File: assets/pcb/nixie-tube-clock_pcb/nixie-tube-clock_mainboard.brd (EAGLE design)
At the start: 90.2 x 40.6 mm, 14 parts, among them J1 POW (5V), P1 MX, P2 MXX, P3 HX, P4 HXX, P7 RTC, P8 HV_EN

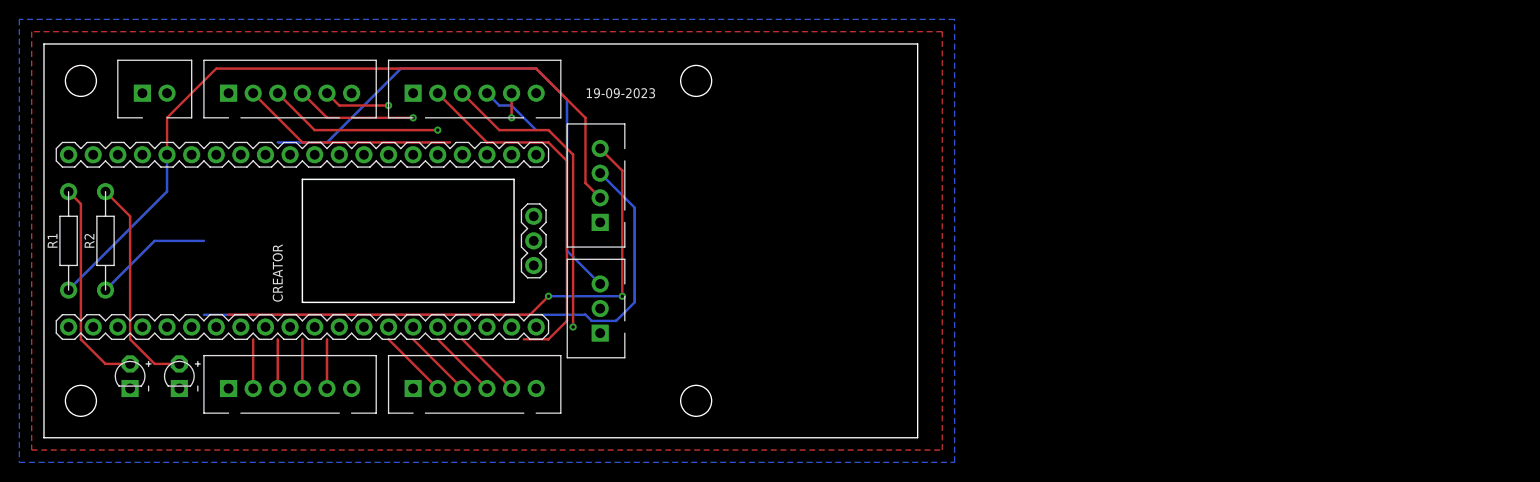
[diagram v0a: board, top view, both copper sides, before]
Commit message: cleaned up files
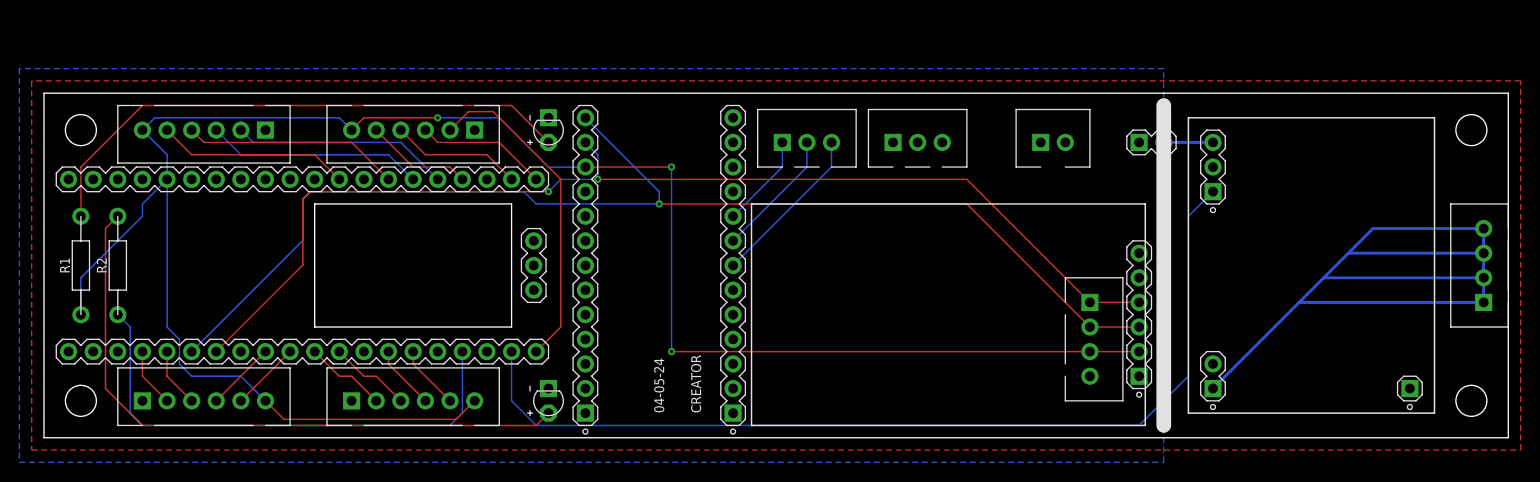
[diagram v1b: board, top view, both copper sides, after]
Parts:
- added GND: GND, myLibrary:XH2.54_3-PIN
- added JP1: (no value), myLibrary:HEADER_2-PIN_JUMPER
- added P11: CAP1188, myLibrary:HEADER_13-PIN
- added P12: (no value), myLibrary:HEADER_13-PIN
- added P5: RTC_A, myLibrary:HEADER_6-PIN
- added P6: HV_OUT, myLibrary:HEADER_2-PIN
- added P9: HV_OUT, myLibrary:XH2.54_4-PIN
- added RTC_B: RTC_B, myLibrary:XH2.54_4-PIN
- added TOUCH: TOUCH, myLibrary:XH2.54_3-PIN
- CREATOR: value Isaac -> ISAAC
- P1: value MX -> MXX
- P2: value MXX -> MX
- P3: value HX -> HXX
- P4: value HXX -> HX
- P7: value RTC -> HV_IN; device myLibrary:XH2.54_4-PIN -> myLibrary:HEADER_3-PIN
- P8: value HV_EN -> (none); device myLibrary:XH2.54_3-PIN -> myLibrary:HEADER_1-PIN
- SCHEMATIC1: value 19-09-2023 -> 04-05-24
- moved J1 92.8 mm to (104.1, 30.5)
- moved P8 84.0 mm to (141.0, 5.08), turned to 0 degrees
- moved P7 63.2 mm to (120.7, 25.4), turned to 0 degrees
- moved LED1 50.1 mm to (52.1, 31.8), turned to 90 degrees
- moved CREATOR 46.7 mm to (68.6, 2.54)
- moved LED2 38.2 mm to (52.1, 3.81), turned to 90 degrees
- moved SCHEMATIC1 34.7 mm to (61.0, 2.54), turned to 90 degrees
- moved P3 28.2 mm to (16.5, 31.8), turned to 180 degrees
- moved P4 13.3 mm to (38.1, 31.8), turned to 180 degrees
- moved P1 8.98 mm to (16.5, 3.81)
- moved P2 6.48 mm to (38.1, 3.81)
- moved R2 2.84 mm to (7.62, 17.8)
- moved R1 2.84 mm to (3.81, 17.8)
- moved MC1 2.54 mm to (26.7, 17.8)
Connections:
- removed net HV_EN: P8.3
- removed net N$3: MC1.6
- removed net N$4: MC1.7
- removed net N$5: MC1.4
- removed net N$6: MC1.5
- removed net N$7: MC1.9
- removed net N$8: MC1.10
- new net 32K: P5.6
- new net BUZZ: MC1.16
- new net C1: P12.9, TOUCH.1
- new net C2: P12.8, TOUCH.2
- new net C3: P12.7, TOUCH.3
- new net C4: P12.6
- new net C5: P12.5
- new net C6: P12.4
- new net C7: P12.3
- new net C8: P12.2
- new net HV: P6.1, P9.1, P9.2, P9.3, P9.4
- new net N$9: JP1.2, P7.3
- new net SHDN: MC1.19, P7.1
- new net SQW: P5.5
- net +3V3: now also P11.11, P5.2, RTC_B.3; no longer P7.2
- net +5V: now also JP1.1; no longer P8.1
- net ACT: now also MC1.17
- net AHX: now also MC1.20, P4.2; no longer P3.2
- net AHXX: now also MC1.25, P3.2; no longer P4.2
- net AMX: now also MC1.11, P2.2; no longer P1.2
- net AMXX: now also MC1.4, P1.2; no longer P2.2
- net BHX: now also MC1.21, P4.3; no longer P3.3
- net BHXX: now also MC1.26, P3.3; no longer P4.3
- net BMX: now also MC1.12, P2.3; no longer P1.3
- net BMXX: now also MC1.5, P1.3; no longer P2.3
- net CHX: now also MC1.22, P4.4; no longer P3.4
- net CHXX: now also MC1.27, P3.4; no longer P4.4
- net CMX: now also MC1.14, P2.4; no longer P1.4
- net CMXX: now also MC1.9, P1.4; no longer P2.4
- net DHX: now also MC1.24, P4.5; no longer P3.5
- net DHXX: now also MC1.29, P3.5; no longer P4.5
- net DMX: now also MC1.15, P2.5; no longer P1.5
- net DMXX: now also MC1.10, P1.5; no longer P2.5
- net GND: now also GND.1, GND.2, GND.3, P11.10, P5.1, P6.2, P7.2, RTC_B.4; no longer P7.1, P8.2
- net SCL: now also MC1.7, P11.12, P5.4, RTC_B.1; no longer P7.4
- net SDA: now also MC1.6, P11.13, P5.3, RTC_B.2; no longer P7.3
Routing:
- net +3V3: track 78.3 -> 202.6 mm, vias 0 -> 3
- net SHDN: track 0.00 -> 98.2 mm
- net HV: track 0.00 -> 91.9 mm
- net SDA: track 60.3 -> 125.0 mm, vias 0 -> 1
- net SCL: track 57.6 -> 116.2 mm
- net HV_EN: track 54.8 -> 0.00 mm
- net N$2: track 22.4 -> 66.1 mm
- net ACT: track 12.3 -> 52.4 mm
- net N$1: track 21.9 -> 57.5 mm
- net BHX: track 31.8 -> 13.5 mm, vias 1 -> 0
- net C3: track 0.00 -> 16.9 mm
- net C2: track 0.00 -> 13.3 mm
- net DHXX: track 6.88 -> 19.9 mm, vias 1 -> 0
- net CHXX: track 12.5 -> 22.4 mm, vias 1 -> 0
- net C1: track 0.00 -> 9.72 mm
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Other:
- board size 90.2 x 40.6 mm -> 151.1 x 35.6 mm
